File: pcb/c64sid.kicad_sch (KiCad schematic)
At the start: 10 parts, among them U1 PCF8574A, U2 LM386, U3 MOS6581, U4 ESP32-S2-SAOLA-1R

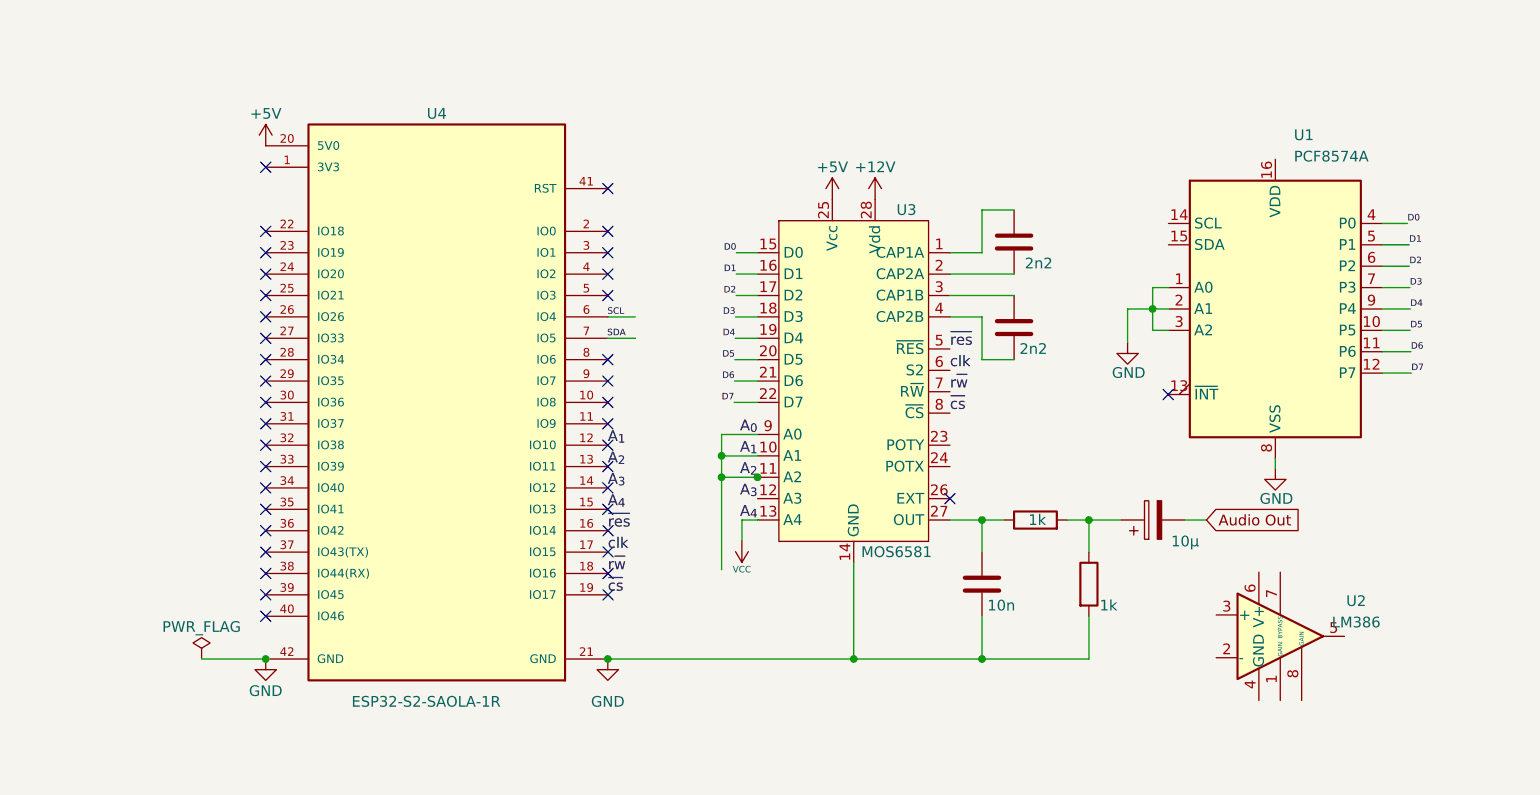
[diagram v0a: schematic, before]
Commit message: Proef commit
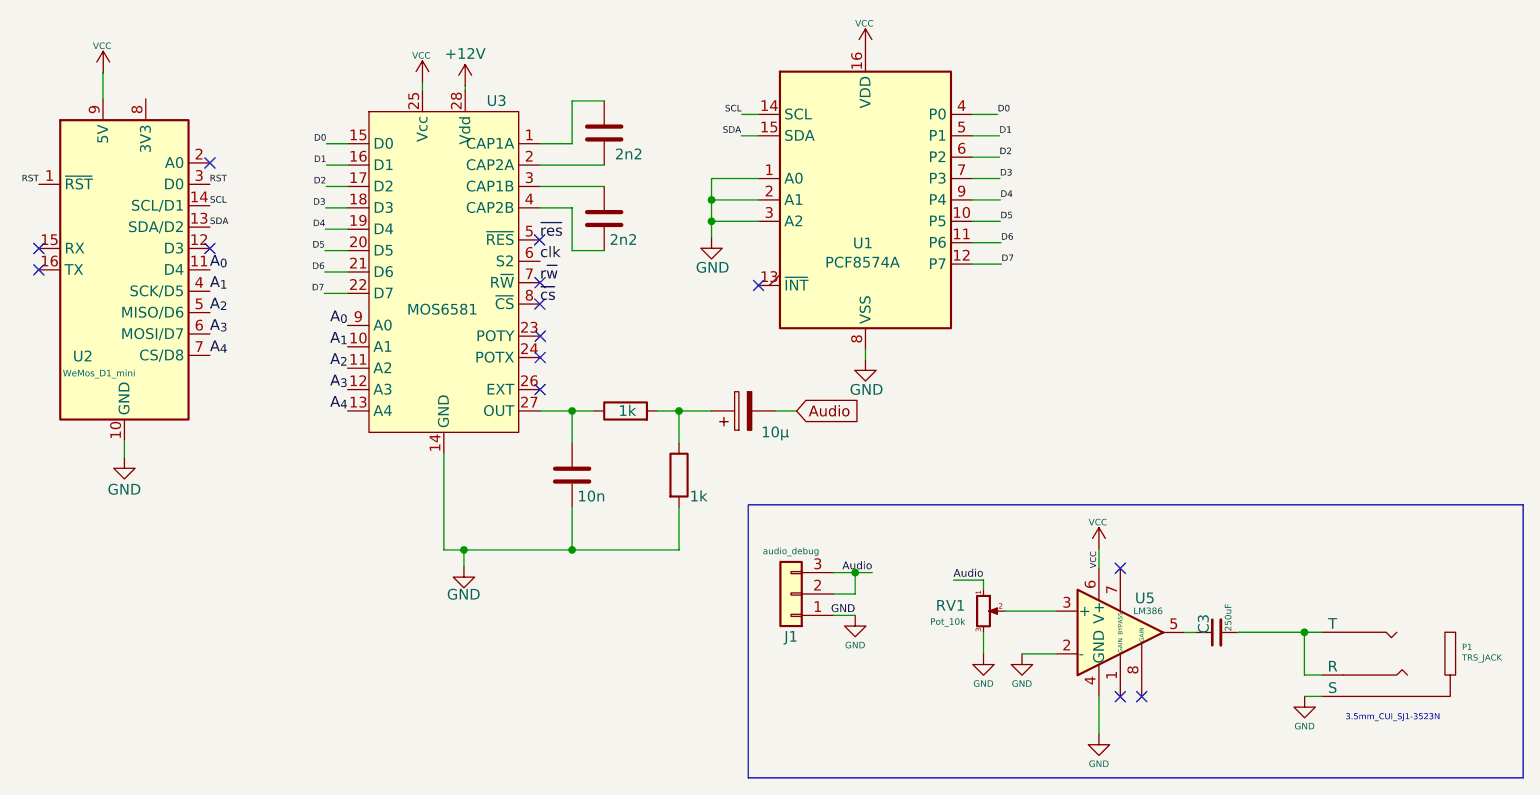
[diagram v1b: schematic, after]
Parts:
- removed U2: LM386, symbol Amplifier_Audio:LM386
- removed U4: ESP32-S2-SAOLA-1R, XCVR_ESP32-S2-SAOLA-1R, symbol parts:ESP32-S2-SAOLA-1R
- added C3: 250uF, Capacitor_THT:C_Disc_D3.4mm_W2.1mm_P2.50mm, symbol Device:C_Small
- added J1: audio_debug, Connector_PinHeader_2.54mm:PinHeader_1x03_P2.54mm_Vertical, symbol SN76849 Arduino nano shield-rescue:Conn_01x03-conn
- added P1: TRS_JACK, Connector_Audio:Jack_3.5mm_CUI_SJ1-3523N_Horizontal, symbol trs_jack:TRS_JACK
- added RV1: Pot_10k, Potentiometer_THT:Potentiometer_Bourns_3339P_Vertical, symbol Device:R_Potentiometer_Small
- added U2: WeMos_D1_mini, Module:WEMOS_D1_mini_light, symbol MCU_Module:WeMos_D1_mini
- added U5: LM386, Package_DIP:DIP-8_W7.62mm, symbol Amplifier_Audio:LM386
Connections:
- net +5V is gone; now on net VCC: U3.25 (Vcc)
- net A_{0}: now also U2.11 (D4); no longer U3.10 (A1), U3.11 (A2)
- net A_{3}: now also U2.6 (MOSI/D7)
- net A_{4}: now also U2.7 (CS/D8)
- net GND: now also U1.2 (A1), U1.3 (A2), J1.1 (Pin_1), P1.1 (S), RV1.3, U2.10 (GND), U5.2 (-), U5.4 (GND); no longer U3.14 (GND)
- net SCL: now also U1.14 (SCL), U2.14 (SCL/D1)
- net SDA: now also U1.15 (SDA), U2.13 (SDA/D2)
- net VCC: now also U1.16 (VDD), U2.9 (5V), U5.6 (V+)
- net Audio Out renamed Audio
- net Audio: now also J1.2 (Pin_2), J1.3 (Pin_3), RV1.1
- new net: RV1.2, U5.3 (+)
- new net: C3.1, U5.5
- new net: C3.2, P1.2 (T), P1.3 (R)
- new net A_{1}: U2.4 (SCK/D5), U3.10 (A1)
- new net A_{2}: U2.5 (MISO/D6), U3.11 (A2)
- new net RST: U2.1 (~{RST})
- no-connect marks 39 -> 14
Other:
- note added: "3.5mm_CUI_SJ1-3523N"
- company: (none) -> Easylab4kids & Michiel Erasmus
- title: (none) -> ESP32 SID player voor Commodore 64 
- moved on the sheet: U1, U3
